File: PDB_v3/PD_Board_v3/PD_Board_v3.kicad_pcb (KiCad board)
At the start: 2 copper layers, 28 x 33.2 mm, 6 parts, among them J1 Wepon, J2 Servo, J3 Batt, J4 Drive_pwr, J5 Recv, J7 Drive_Sig/5v

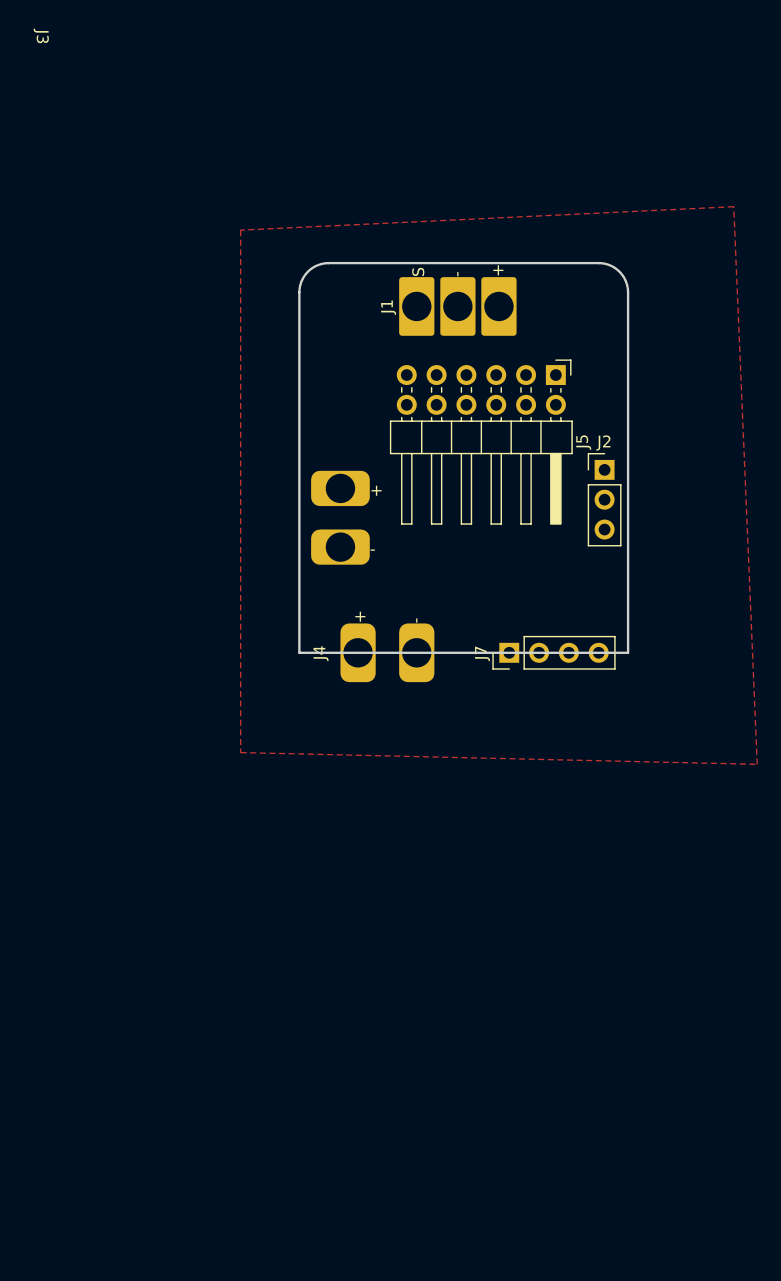
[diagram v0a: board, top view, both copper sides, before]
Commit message: inital route
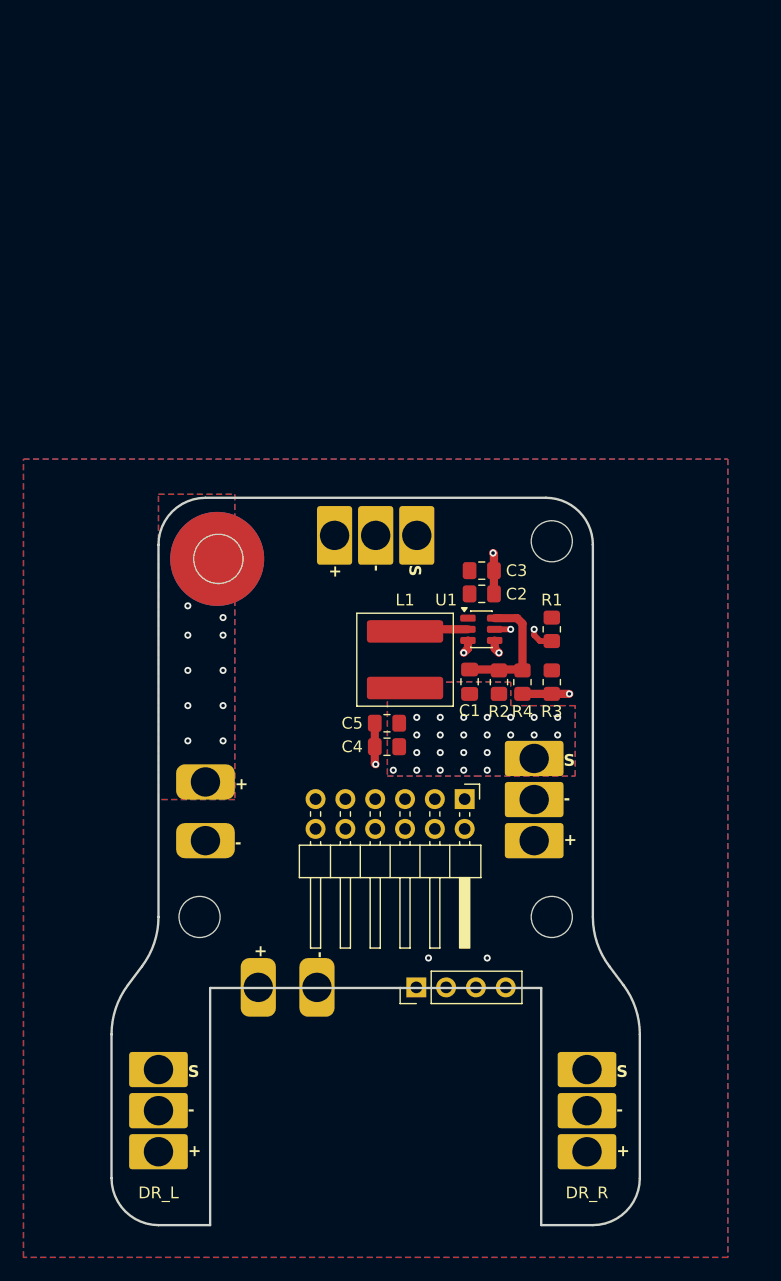
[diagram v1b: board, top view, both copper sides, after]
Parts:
- added C1: 33pF, Capacitor_SMD:C_0805_2012Metric_Pad1.18x1.45mm_HandSolder, F.Cu at (151.5, 63.5)
- added C2: 10uF, Capacitor_SMD:C_0805_2012Metric_Pad1.18x1.45mm_HandSolder, F.Cu at (152.5, 56.0)
- added C3: 100nF, Capacitor_SMD:C_0805_2012Metric_Pad1.18x1.45mm_HandSolder, F.Cu at (152.5, 54.0)
- added C4: 47uF, Capacitor_SMD:C_0805_2012Metric_Pad1.18x1.45mm_HandSolder, F.Cu at (144.5, 69.0)
- added C5: 100nF, Capacitor_SMD:C_0805_2012Metric_Pad1.18x1.45mm_HandSolder, F.Cu at (144.5, 67.0)
- added H1: MountingHole, MountingHole:MountingHole_3.5mm, F.Cu at (158.5, 51.5)
- added H3: MountingHole, MountingHole:MountingHole_3.5mm, F.Cu at (158.5, 83.5)
- added H4: MountingHole, MountingHole:MountingHole_3.5mm, F.Cu at (128.5, 83.5)
- added J6: Drive_pwr, Connectors:XT30, F.Cu at (133.5, 89.5)
- added J8: DR_L, Connectors:MR30, F.Cu at (125.0, 96.5)
- added J9: DR_R, Connectors:MR30, F.Cu at (161.5, 96.5)
- added L1: 3.3uH, Inductor_SMD:L_Coilcraft_XAL7070-XXX, F.Cu at (146.0, 61.6)
- added R1: 100k, Resistor_SMD:R_0805_2012Metric_Pad1.20x1.40mm_HandSolder, F.Cu at (158.5, 59.0)
- added R2: 270k, Resistor_SMD:R_0805_2012Metric_Pad1.20x1.40mm_HandSolder, F.Cu at (154.0, 63.5)
- added R3: 12.1k, Resistor_SMD:R_0805_2012Metric_Pad1.20x1.40mm_HandSolder, F.Cu at (158.5, 63.5)
- added R4: 30k, Resistor_SMD:R_0805_2012Metric_Pad1.20x1.40mm_HandSolder, F.Cu at (156.0, 63.5)
- added U1: ~, Package_TO_SOT_SMD:SOT-23-6, F.Cu at (152.5, 59.0)
- J2: value Servo -> Batt; footprint Connector_PinHeader_2.54mm:PinHeader_1x03_P2.54mm_Vertical -> Connectors:XT30
- J3: value Batt -> SW; footprint Connectors:XT30 -> Project:SMD_SW
- J4: value Drive_pwr -> Drive_Sig/5v; footprint Connectors:XT30 -> Connector_PinHeader_2.54mm:PinHeader_1x04_P2.54mm_Vertical
- J7: value Drive_Sig/5v -> Servo; footprint Connector_PinHeader_2.54mm:PinHeader_1x04_P2.54mm_Vertical -> Connectors:MR30
- moved J2 43.2 mm to (129.0, 72.0)
- moved J5 36.9 mm to (151.1, 73.5)
- moved J4 28.9 mm to (147.0, 89.5)
- moved J1 19.5 mm to (147.0, 51.0), turned to -90 degrees
- moved J3 12.1 mm to (130.0, 53.0)
- moved J7 9.25 mm to (157.0, 70.0), turned to 0 degrees
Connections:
- J1 pad 1: Net-(J1-Pin_1) -> +BATT_SW
- J1 pad 2: Net-(J1-Pin_2) -> /S2
- J1 pad 3: /BATT+ -> GND
- J2 pad 1: Net-(J2-Pin_1) -> +BATT
- J2 pad 2: unconnected-(J2-Pin_2-Pad2) -> GND
- J3 pad 1: Net-(J3-Pin_1) -> +BATT
- J3 pad 2: /BATT+ -> +BATT_SW
- J4 pad 1: /BATT+ -> GND
- J4 pad 2: Net-(J1-Pin_2) -> +5V
- J5 pad 1: Net-(J5-Pin_1) -> /S1
- J5 pad 10: unconnected-(J5-Pin_10-Pad10) -> GND
- J5 pad 11: unconnected-(J5-Pin_11-Pad11) -> +5V
- J5 pad 12: Net-(J2-Pin_1) -> /S4
- J5 pad 2: unconnected-(J5-Pin_2-Pad2) -> +5V
- J5 pad 3: unconnected-(J5-Pin_3-Pad3) -> GND
- J5 pad 4: Net-(J5-Pin_4) -> GND
- J5 pad 5: Net-(J5-Pin_5) -> +5V
- J5 pad 6: Net-(J5-Pin_6) -> /S2
- J5 pad 7: Net-(J1-Pin_1) -> /S3
- J5 pad 8: unconnected-(J5-Pin_8-Pad8) -> +5V
- J5 pad 9: unconnected-(J5-Pin_9-Pad9) -> GND
- J7 pad 1: Net-(J5-Pin_4) -> +6V
- J7 pad 2: Net-(J5-Pin_5) -> /S1
- J7 pad 3: Net-(J5-Pin_1) -> GND
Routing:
- net +5V: track 0.00 -> 30.2 mm
- net /S4: track 0.00 -> 25.9 mm, vias 0 -> 2
- net /S2: track 0.00 -> 24.6 mm
- net GND: track 0.00 -> 13.4 mm, vias 0 -> 5
- net /S3: track 0.00 -> 13.4 mm
- net Net-(U1-FB): track 0.00 -> 10.6 mm
- net /S1: track 0.00 -> 7.02 mm
- net Net-(U1-EN): track 0.00 -> 5.57 mm, vias 0 -> 2
- net Net-(U1-SW): track 0.00 -> 5.44 mm
- net +BATT: vias 0 -> 10
- net +6V: vias 0 -> 23
- added copper zone on B.Cu, net +6V
- added copper zone on F.Cu, net +6V
- added copper zone on In1.Cu, net +6V
- added copper zone on In2.Cu, net +6V
- added copper zone on B.Cu, net +BATT
- added copper zone on F.Cu, net +BATT
- added copper zone on In1.Cu, net +BATT
- added copper zone on In2.Cu, net +BATT
- added copper zone on F.Cu, net +BATT_SW
- added copper zone on B.Cu, net GND
- removed copper zone on F.Cu, net /BATT+
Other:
- board size 28 x 33.2 mm -> 45 x 62 mm
- copper layers 2 -> 4

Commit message: almost done
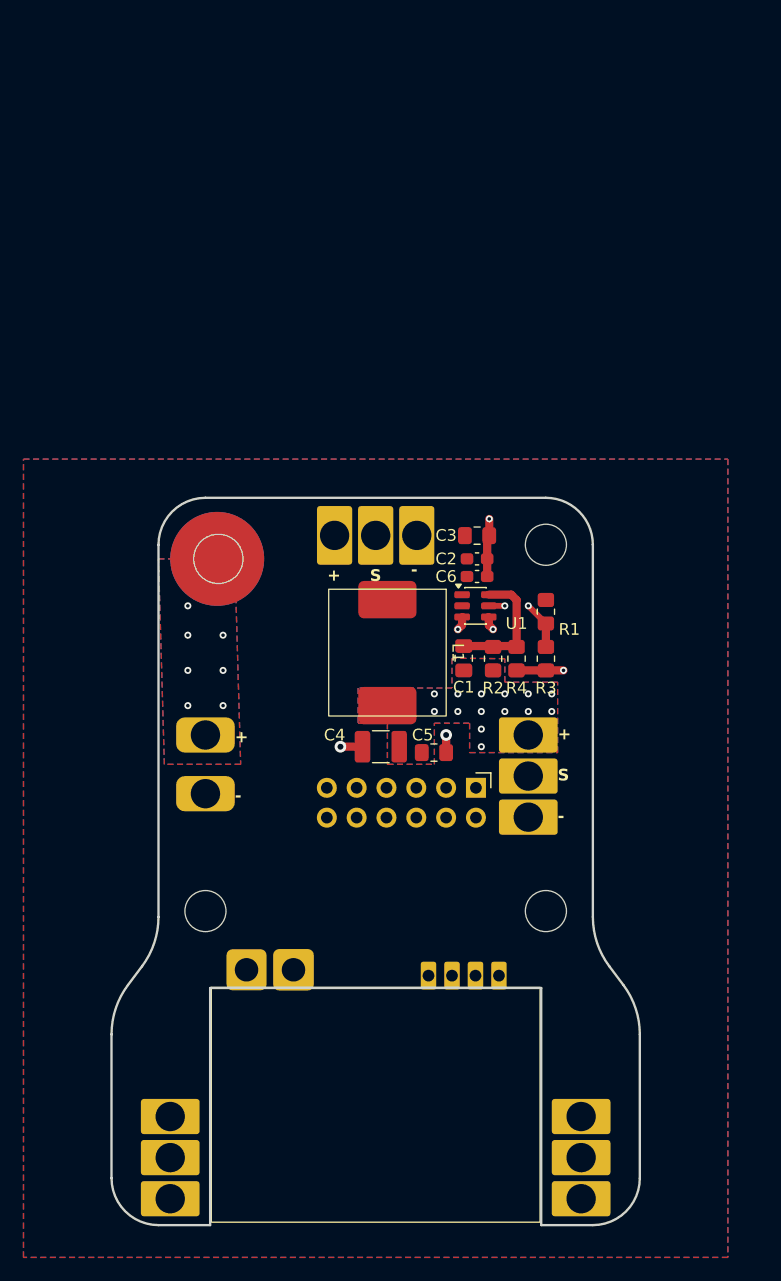
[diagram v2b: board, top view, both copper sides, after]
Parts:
- removed J4: Drive_Sig/5v, Connector_PinHeader_2.54mm:PinHeader_1x04_P2.54mm_Vertical
- removed J6: Drive_pwr, Connectors:XT30
- removed J8: DR_L, Connectors:MR30
- removed J9: DR_R, Connectors:MR30
- added C6: 10uF, Capacitor_SMD:C_0603_1608Metric_Pad1.08x0.95mm_HandSolder, F.Cu at (152.1, 54.5)
- added E1: Dual_ESC, Project:Dual_ESC, F.Cu at (143.5, 99.5)
- C2: footprint Capacitor_SMD:C_0805_2012Metric_Pad1.18x1.45mm_HandSolder -> Capacitor_SMD:C_0603_1608Metric_Pad1.08x0.95mm_HandSolder
- C4: footprint Capacitor_SMD:C_0805_2012Metric_Pad1.18x1.45mm_HandSolder -> Capacitor_SMD:C_1210_3225Metric_Pad1.33x2.70mm_HandSolder
- L1: footprint Inductor_SMD:L_Coilcraft_XAL7070-XXX -> Project:Inductor
- moved J1 7.00 mm to (140.0, 51.0), turned to 90 degrees
- moved C5 4.72 mm to (148.5, 69.5), turned to 0 degrees
- moved J2 4.00 mm to (129.0, 68.0)
- moved C2 3.01 mm to (152.1, 53.0)
- moved C3 3.01 mm to (152.1, 51.0)
- moved C1 2.06 mm to (151.0, 61.5)
- moved J7 2.06 mm to (156.5, 68.0)
- moved R2 2.06 mm to (153.5, 61.5)
- moved R3 2.06 mm to (158.0, 61.5)
- moved R4 2.06 mm to (155.5, 61.5)
- moved U1 2.06 mm to (152.0, 57.0)
- moved L1 1.62 mm to (144.5, 61.0)
- moved R1 1.58 mm to (158.0, 57.5)
- moved J5 1.36 mm to (152.0, 72.5)
- moved H3 0.71 mm to (158.0, 83.0)
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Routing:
- net /S3: track 13.4 -> 0.11 mm
- net +5V: track 30.2 -> 17.9 mm
- net /S1: track 7.02 -> 0.06 mm
- net Net-(U1-SW): track 5.44 -> 0.00 mm
- net /S4: track 25.9 -> 21.0 mm, vias 2 -> 0
- net Net-(U1-EN): track 5.57 -> 7.48 mm
- net +6V: track 0.00 -> 1.41 mm, vias 23 -> 14
- net GND: track 13.4 -> 14.8 mm, vias 5 -> 6
- net /S2: track 24.6 -> 23.9 mm
- net +BATT: vias 10 -> 7
